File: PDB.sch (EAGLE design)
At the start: 79 parts

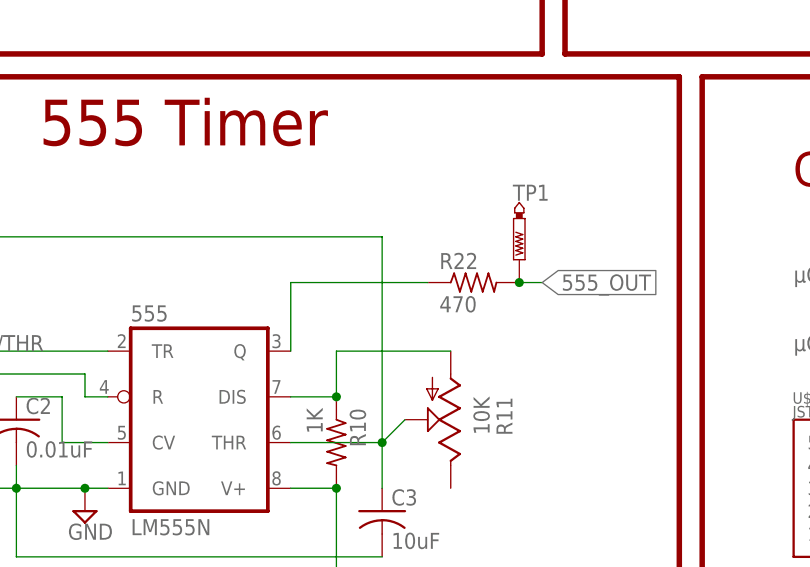
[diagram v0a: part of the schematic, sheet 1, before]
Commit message: PCB layout
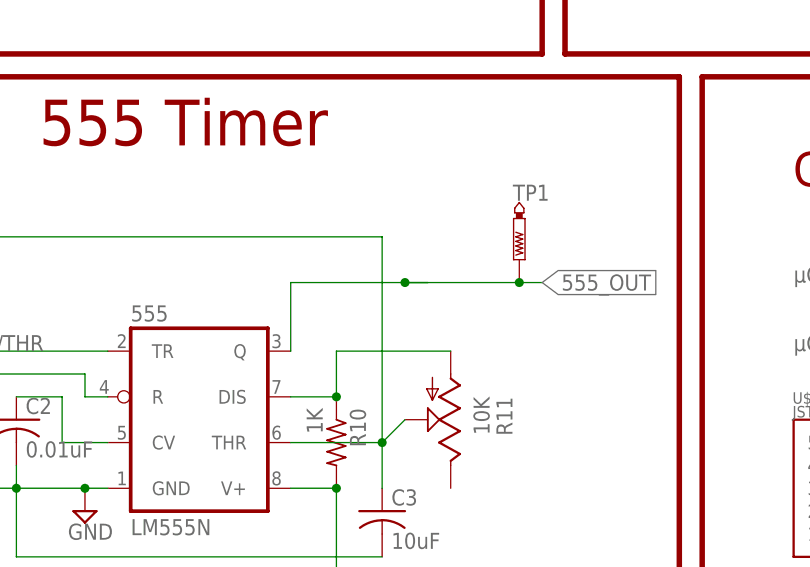
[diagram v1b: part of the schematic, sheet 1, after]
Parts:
- removed R22: 470, rcl:R-US_R3225
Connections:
- removed net Q: 555.Q, R22.1
- net 555_OUT: now also 555.Q; no longer R22.2
